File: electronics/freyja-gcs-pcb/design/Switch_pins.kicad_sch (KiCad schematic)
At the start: 23 parts, among them J5 XT60PB-M.G.Y, SW3 TS1210CJ 250GF 009, U4 ST-0-102-A01-T000-LF+PJ, U5 ST-0-102-A01-T000-LF+PJ, U6 ST-0-102-A01-T000-LF+PJ, U7 ST-0-102-A01-T000-LF+PJ, U8 ST-0-102-A01-T000-LF+PJ, U9 ST-0-102-A01-T000-LF+PJ

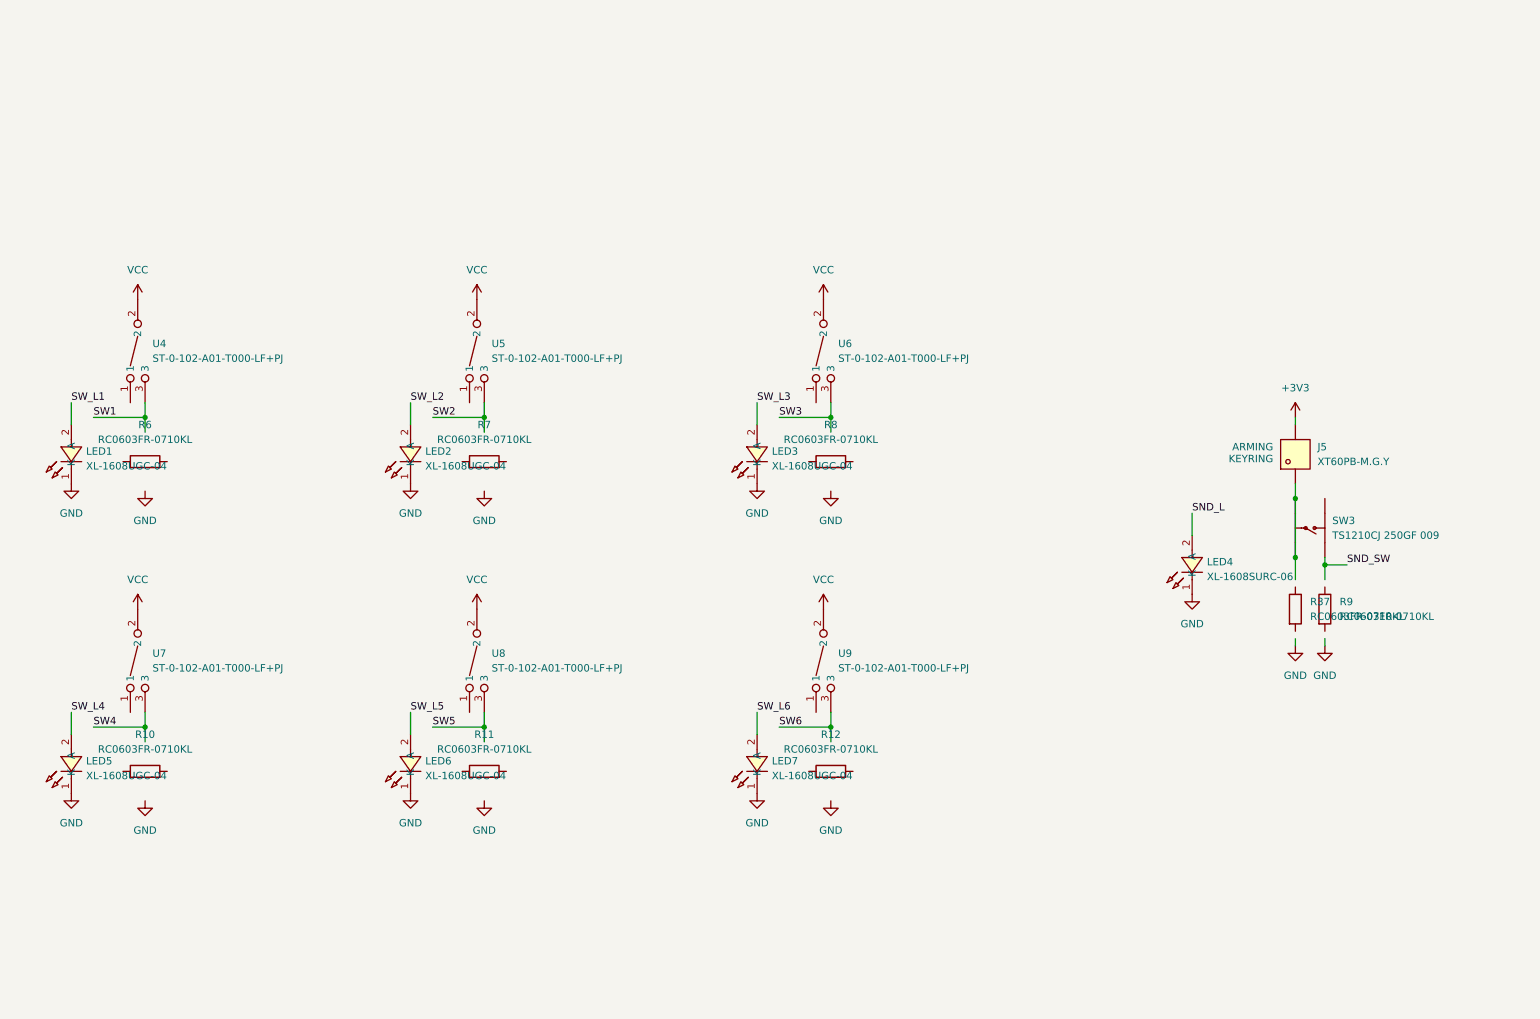
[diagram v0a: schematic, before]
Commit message: buttons and indicators
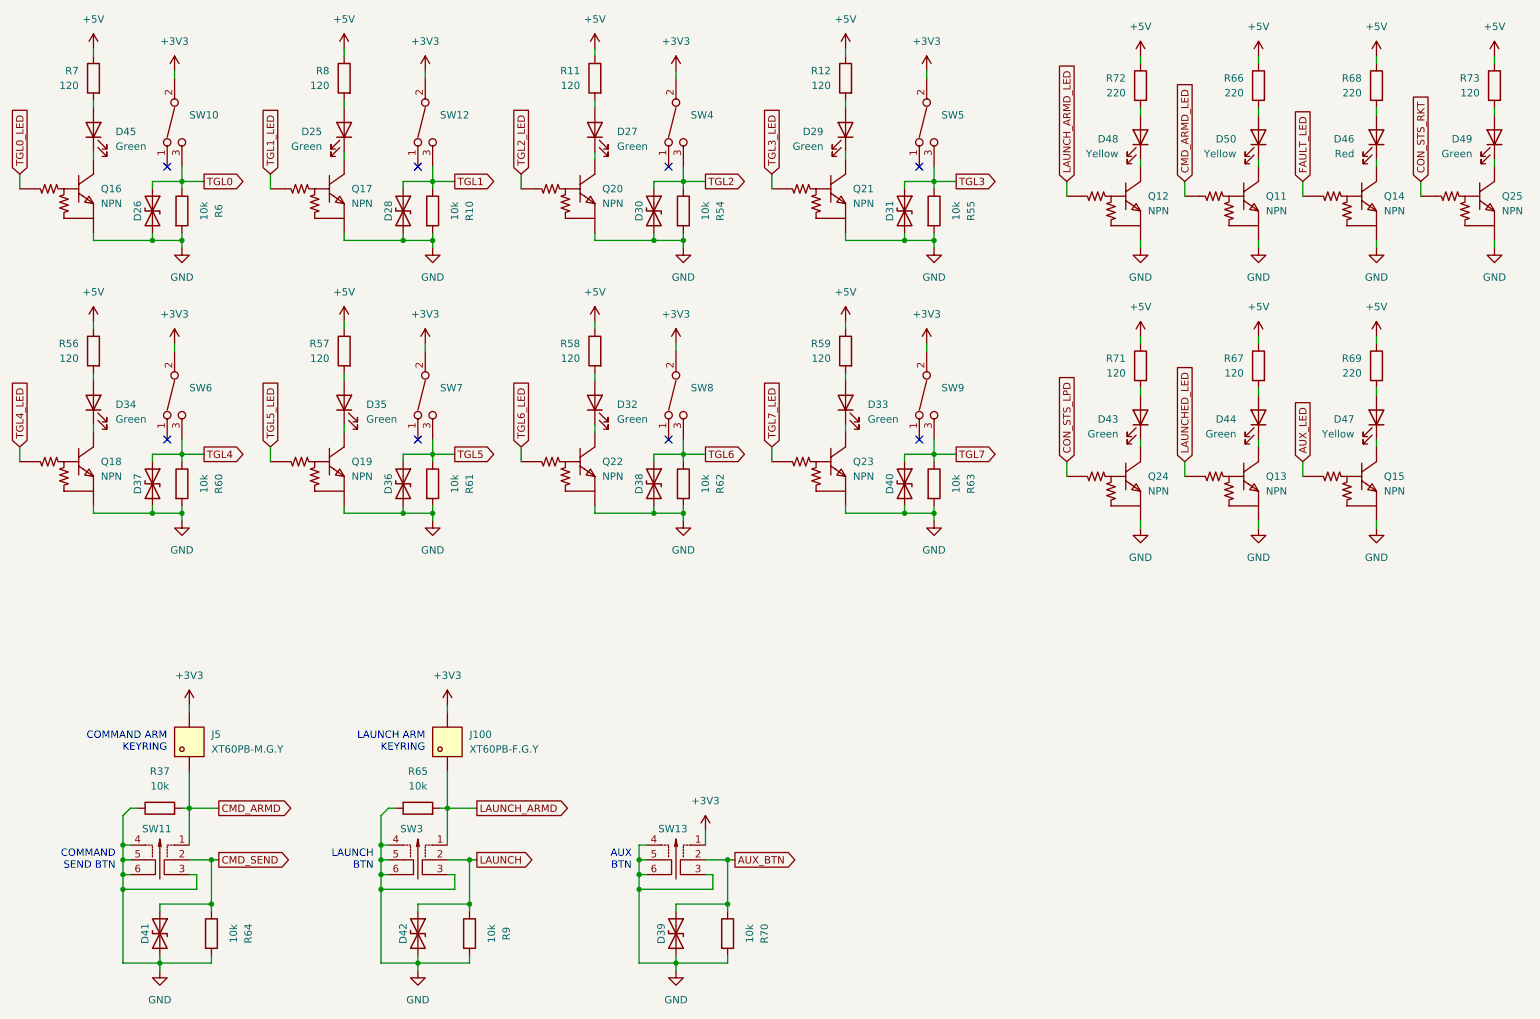
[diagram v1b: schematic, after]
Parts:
- removed LED1, LED2, LED3, LED5, LED6, LED7: XL-1608UGC-04, EasyEDA:LED0603-RD_GREEN, symbol EasyEDA:XL-1608UGC-04
- removed LED4: XL-1608SURC-06, EasyEDA:LED0603-RD_RED, symbol EasyEDA:XL-1608SURC-06
- removed SW3: TS1210CJ 250GF 009, EasyEDA:SW-TH_4P-L12.0-W12.0-P5.00-LS12.5_TC-1103XX, symbol EasyEDA:TS1210CJ250GF009
- removed U5, U6, U7, U8, U9: ST-0-102-A01-T000-LF+PJ, EasyEDA:SW-TH_3P-L8.3-W5.2-P2.54_ST-0-102-A01-T000, symbol EasyEDA:ST-0-102-A01-T000-LF+PJ
- added D25, D27, D29, D32, D33, D34, D35, D43, D44, D45, D49: Green, EasyEDA:LED-TH_BD5.9-P2.54-RD_GREEN, symbol Device:LED
- added D26, D28, D30, D31, D36, D37, D38, D39, D40, D41, D42: 0603ESDA-05N, Diode_SMD:D_0603_1608Metric_Pad1.05x0.95mm_HandSolder, symbol Device:D_TVS
- added D46: Red, EasyEDA:LED-TH_BD5.9-P2.54-RD_GREEN, symbol Device:LED
- added D47, D48, D50: Yellow, EasyEDA:LED-TH_BD5.9-P2.54-RD_GREEN, symbol Device:LED
- added J100: XT60PB-F.G.Y, EasyEDA:CONN-TH_XT60PB-M, symbol EasyEDA:XT60PB-M.G.Y
- added Q11, Q12, Q13, Q14, Q15, Q16, Q17, Q18, Q19, Q20, Q21, Q22, Q23, Q24, Q25: NPN, EasyEDA:SOT-416_L1.6-W0.8-P1.00-LS1.6-BR, symbol EasyEDA:DTC043ZEBTL
- added R54, R55, R60, R61, R62, R63, R64, R65, R70: 10k, EasyEDA:R0603, symbol Device:R
- added R56, R57, R58, R59, R67, R71, R73: 120, symbol Device:R
- added R66, R68, R69, R72: 220, symbol Device:R
- added SW11, SW13, SW3: PB22E09071, EasyEDA:SW-TH_6P-L8.5-W8.5-P2.54-LS5.5, symbol EasyEDA:PB22E09071
- added SW12, SW4, SW5, SW6, SW7, SW8, SW9: ST-0-102-A01-T000-LF+PJ, EasyEDA:SW-TH_3P-L8.3-W5.2-P2.54_ST-0-102-A01-T000, symbol EasyEDA:ST-0-102-A01-T000-LF+PJ
- R10, R37, R6, R9: value RC0603FR-0710KL -> 10k
- R11, R12, R7, R8: value RC0603FR-0710KL -> 120; footprint EasyEDA:R0603 -> (none); LCSC Part C98220 -> (none)
- renumbered U4 to SW10
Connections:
- net SW1 is gone; now on net TGL0: SW10.3
- net VCC is gone; now on net +3V3: SW10.2
- net +3V3: now also J100.2, SW12.2, SW13.1, SW4.2, SW5.2, SW6.2, SW7.2, SW8.2, SW9.2
- net GND: now also R10.2, R37.1, R6.2, R9.2, D26.2 (A2), D28.2 (A2), D30.2 (A2), D31.2 (A2), D36.2 (A2), D37.2 (A2), D38.2 (A2), D39.2 (A2), D40.2 (A2), D41.2 (A2), D42.2 (A2), Q11.2 (E), Q12.2 (E), Q13.2 (E), Q14.2 (E), Q15.2 (E), Q16.2 (E), Q17.2 (E), Q18.2 (E), Q19.2 (E), Q20.2 (E), Q21.2 (E), Q22.2 (E), Q23.2 (E), Q24.2 (E), Q25.2 (E), R54.2, R55.2, R60.2, R61.2, R62.2, R63.2, R64.2, R65.1, R70.2, SW11.3, SW11.4, SW11.5, SW11.6, SW13.3, SW13.4, SW13.5, SW13.6, SW3.3, SW3.4, SW3.5, SW3.6
- net +5V: now reaches R8.1
- net +5V: now also R11.1, R12.1, R7.1, R56.1, R57.1, R58.1, R59.1, R66.1, R67.1, R68.1, R69.1, R71.1, R72.1, R73.1
- net at R8.2: now also D25.2 (A)
- net LAUNCH: now reaches R9.1
- net LAUNCH: now also D42.1 (A1), SW3.2
- net TGL0: now reaches R6.1
- net TGL0: now also D26.1 (A1)
- net CMD_ARMD: now reaches R37.2
- net CMD_ARMD: now also J5.1, SW11.1
- net at R12.2: now also D29.2 (A)
- net at R11.2: now also D27.2 (A)
- net at R7.2: now also D45.2 (A)
- net TGL1: now reaches R10.1
- net TGL1: now also D28.1 (A1), SW12.3
- new net: D43.1 (K), Q24.3 (C)
- new net: D50.2 (A), R66.2
- new net: D48.1 (K), Q12.3 (C)
- new net: D35.1 (K), Q19.3 (C)
- new net: D33.1 (K), Q23.3 (C)
- new net: D33.2 (A), R59.2
- new net: D25.1 (K), Q17.3 (C)
- new net: D29.1 (K), Q21.3 (C)
- new net: D50.1 (K), Q11.3 (C)
- new net: D48.2 (A), R72.2
- new net: D46.2 (A), R68.2
- new net: D47.1 (K), Q15.3 (C)
- new net: D47.2 (A), R69.2
- new net: D34.2 (A), R56.2
- new net: D34.1 (K), Q18.3 (C)
- new net: D49.1 (K), Q25.3 (C)
- new net: D32.1 (K), Q22.3 (C)
- new net: D43.2 (A), R71.2
- new net: D46.1 (K), Q14.3 (C)
- new net: D27.1 (K), Q20.3 (C)
- new net: D44.2 (A), R67.2
- new net: D44.1 (K), Q13.3 (C)
- new net: D32.2 (A), R58.2
- new net: D45.1 (K), Q16.3 (C)
- new net: D35.2 (A), R57.2
- new net: D49.2 (A), R73.2
- new net AUX_BTN: D39.1 (A1), R70.1, SW13.2
- new net AUX_LED: Q15.1 (B)
- new net CMD_ARMD_LED: Q11.1 (B)
- new net CMD_SEND: D41.1 (A1), R64.1, SW11.2
- new net CON_STS_LPD: Q24.1 (B)
- new net CON_STS_RKT: Q25.1 (B)
- new net FAULT_LED: Q14.1 (B)
- new net LAUNCHED_LED: Q13.1 (B)
- new net LAUNCH_ARMD: J100.1, R65.2, SW3.1
- new net LAUNCH_ARMD_LED: Q12.1 (B)
- new net TGL0_LED: Q16.1 (B)
- new net TGL1_LED: Q17.1 (B)
- new net TGL2: D30.1 (A1), R54.1, SW4.3
- new net TGL2_LED: Q20.1 (B)
- new net TGL3: D31.1 (A1), R55.1, SW5.3
- new net TGL3_LED: Q21.1 (B)
- new net TGL4: D37.1 (A1), R60.1, SW6.3
- new net TGL4_LED: Q18.1 (B)
- new net TGL5: D36.1 (A1), R61.1, SW7.3
- new net TGL5_LED: Q19.1 (B)
- new net TGL6: D38.1 (A1), R62.1, SW8.3
- new net TGL6_LED: Q22.1 (B)
- new net TGL7: D40.1 (A1), R63.1, SW9.3
- new net TGL7_LED: Q23.1 (B)
- no-connect marks 0 -> 8
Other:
- note added: "AUX BTN"
- note added: "COMMAND ARM KEYRING"
- note added: "COMMAND SEND BTN"
- note added: "LAUNCH ARM KEYRING"
- note added: "LAUNCH BTN"
- note removed: "ARMING KEYRING"
- moved on the sheet: J5, R6
